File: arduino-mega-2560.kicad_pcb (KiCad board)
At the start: 2 copper layers, 104 x 53.4 mm, 75 parts, among them J1 Conn_02x02_Odd_Even, J10 Conn_01x10, J11 Conn_02x03_Odd_Even, J12 USB_B, J15 Conn_02x03_Odd_Even, J2 PJ-031DH, J4 Conn_02x18_Odd_Even, J5 Conn_01x08, J6 Conn_01x08, J7 Conn_01x08, J8 Conn_01x08, J9 Conn_01x08, SW1 SW_MEC_5E, U1 LMV358, U2 LD1117S50CTR, U3 ATmega16U2-A, U4 MCU-ATMEGA2560-16AU_TQFP100_, U5 LP2985-3.3, U6 PMV48XP, Y1 CSTCE16M9V53-R0, Y2 Crystal

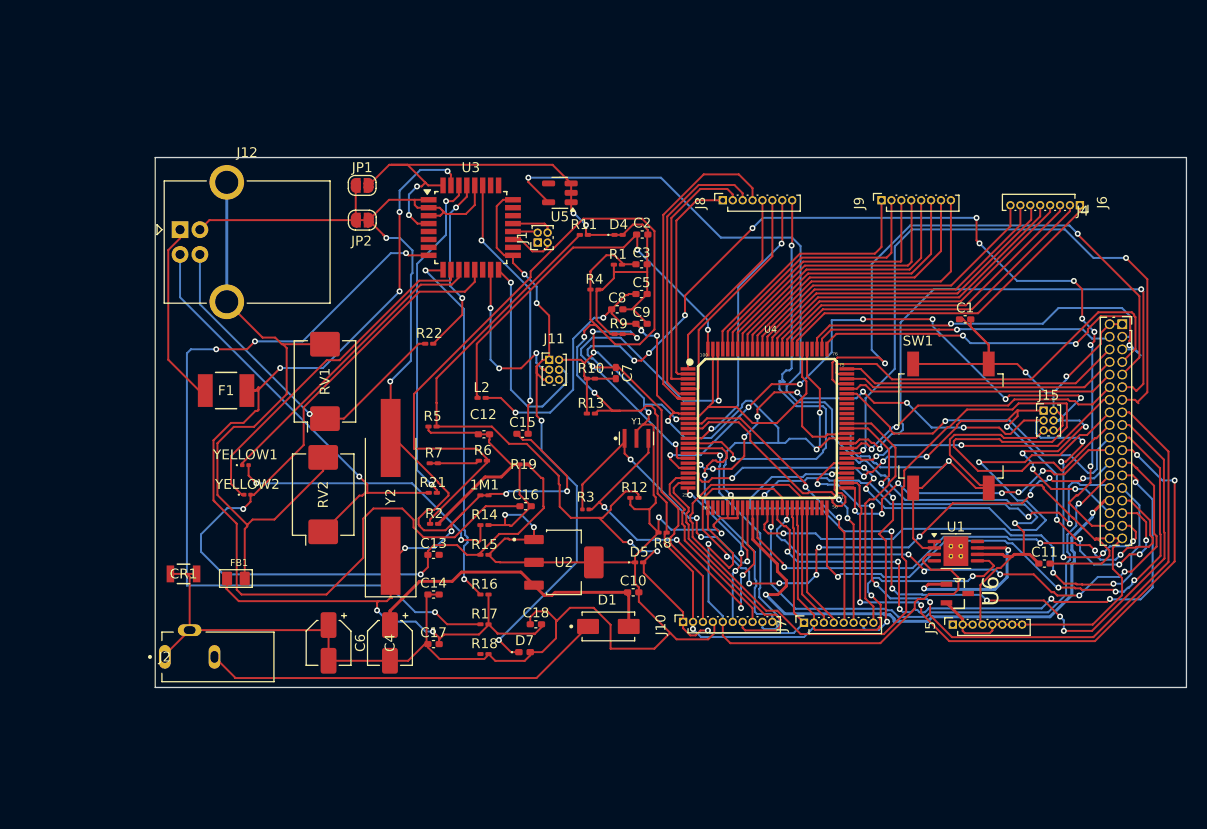
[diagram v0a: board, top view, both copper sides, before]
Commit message: good progress
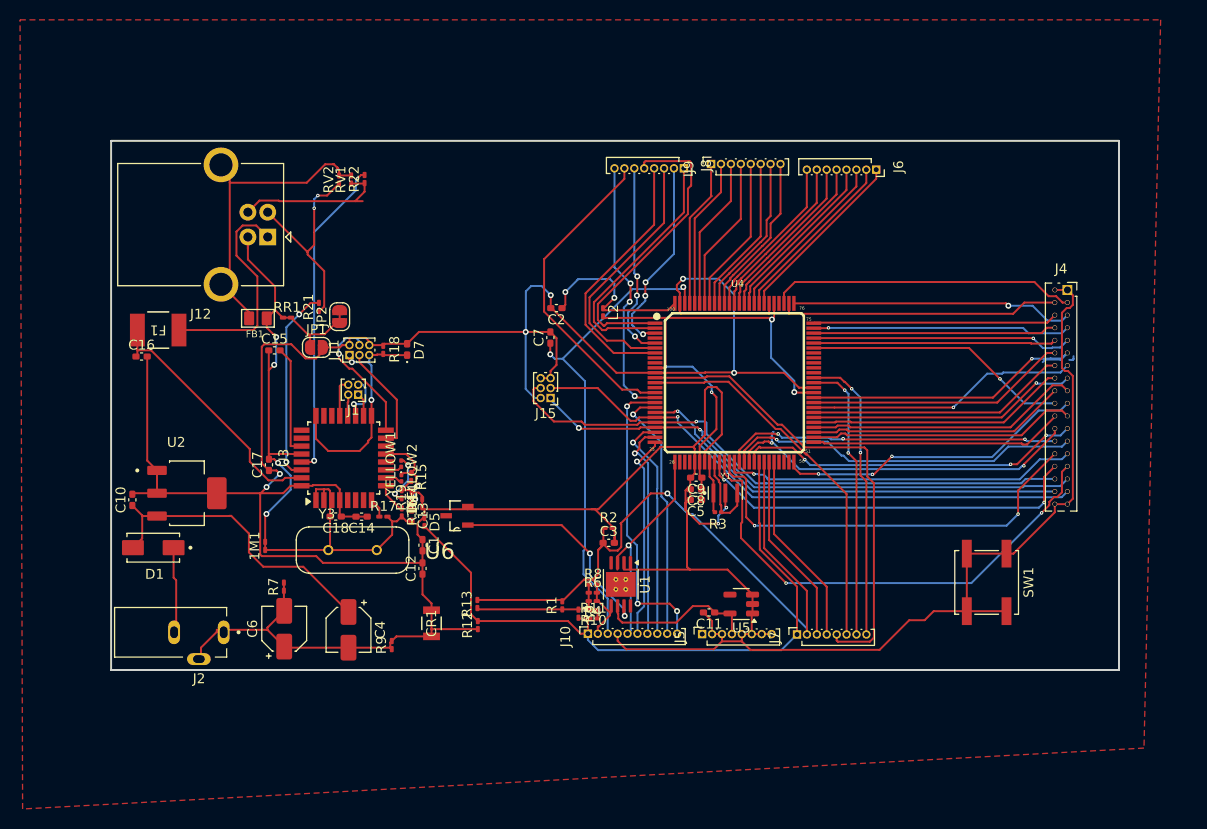
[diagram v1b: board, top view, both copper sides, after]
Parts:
- removed Y2: Crystal, Crystal:Crystal_SMD_HC49-SD_HandSoldering
- added RR1: 1M, Resistor_SMD:R_0201_0603Metric_Pad0.64x0.40mm_HandSolder, F.Cu at (125.1, 90.8)
- added Y3: ECS-160-20-4X-B-DN, ECS_160_20_4X_B_DN:XTAL_ECS-160-20-4X-B-DN, F.Cu at (131.7, 114.3)
- RV1, RV2: footprint Varistor:Varistor_Panasonic_VF -> Resistor_SMD:R_0201_0603Metric_Pad0.64x0.40mm_HandSolder
- SW1: footprint Button_Switch_SMD:SW_MEC_5GSH9 -> Button_Switch_SMD:SW_Push_1P1T_NO_CK_KSC6xxJ
- moved C1 59.3 mm to (138.7, 113.8), turned to -90 degrees
- moved C10 51.3 mm to (109.5, 109.2), turned to 90 degrees
- moved U6 51.0 mm to (142.2, 110.8), turned to 180 degrees
- moved J15 49.7 mm to (151.6, 98.9), turned to 180 degrees
- moved D1 46.6 mm to (111.6, 114.0), turned to 180 degrees
- moved U5 45.3 mm to (170.9, 119.7)
- moved C16 41.5 mm to (110.4, 94.8)
- moved R9 38.8 mm to (135.6, 123.8), turned to 90 degrees
- moved R11 38.7 mm to (156.0, 121.2)
- moved U2 38.6 mm to (115.0, 108.5)
- moved R1 34.8 mm to (152.8, 119.8), turned to 90 degrees
- moved C11 34.2 mm to (167.6, 120.5), turned to 180 degrees
- moved U1 33.9 mm to (158.7, 117.7), turned to -90 degrees
- moved D4 33.5 mm to (138.7, 109.5), turned to 90 degrees
- moved D7 32.7 mm to (137.2, 94.0), turned to 90 degrees
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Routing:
- net /MCU-ATMEGA2560/3: track 180.4 -> 76.1 mm, vias 5 -> 1
- net /MCU-ATMEGA2560/PC0: track 119.7 -> 26.2 mm
- net +3V3: track 102.9 -> 15.2 mm, vias 2 -> 0
- net /ATmega16U2/8: track 83.3 -> 1.99 mm, vias 4 -> 0
- net /ATmega16U2/4: track 89.1 -> 9.92 mm
- net /ATmega16U2/1: track 159.0 -> 81.0 mm, vias 8 -> 4
- net /ATmega16U2/USBVCC: track 100.1 -> 25.6 mm, vias 4 -> 0
- net /MCU-ATMEGA2560/PB0: track 106.6 -> 44.2 mm, vias 12 -> 1
- net /MCU-ATMEGA2560/PC1: track 81.3 -> 27.7 mm, vias 6 -> 0
- net /MCU-ATMEGA2560/PC3: track 71.6 -> 27.3 mm, vias 4 -> 1
- net /MCU-ATMEGA2560/PC5: track 66.5 -> 27.3 mm, vias 2 -> 1
- net +5V: track 490.6 -> 451.8 mm, vias 16 -> 8
- net /MCU-ATMEGA2560/PG1: track 65.1 -> 27.1 mm, vias 4 -> 0
- net /ATmega16U2/MISO2: track 59.2 -> 24.0 mm, vias 4 -> 2
- net Net-(U4-VCC): track 87.6 -> 53.3 mm, vias 8 -> 4
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- added copper zone on F.Cu, net +5V
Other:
- board size 104 x 53.4 mm -> 101.6 x 53.3 mm
